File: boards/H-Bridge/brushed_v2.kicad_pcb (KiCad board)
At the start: 2 copper layers, 58 parts, among them IC1 ISO1042QDWVQ1, IC2 MIC4606-1YML-TR, IC3 AD8410AWBRZ-RL, IC4 TC1108-3.3VDBTR, J1 V+, J2 V-, J3 Motor-, J4 Motor+, J5 CANBus, J6 Encoder, J7 Prog_Header, J8 UART, J9 12V+, Q1 NTBLS4D0N15MC, Q2 NTBLS4D0N15MC, Q3 NTBLS4D0N15MC, Q4 NTBLS4D0N15MC, U1 STM32F103C8Tx, U2 LSF0102DCUR, U3 LSF0102DCUR

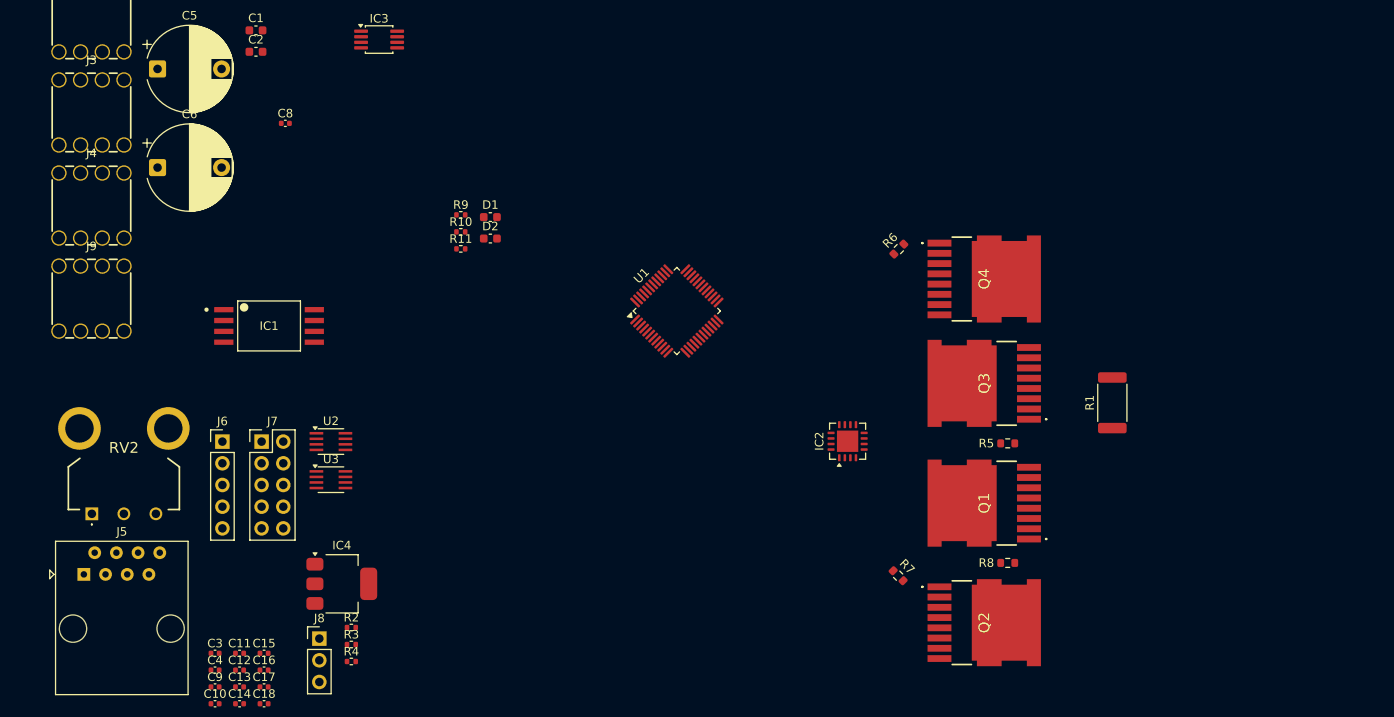
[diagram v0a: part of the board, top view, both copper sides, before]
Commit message: did some layout
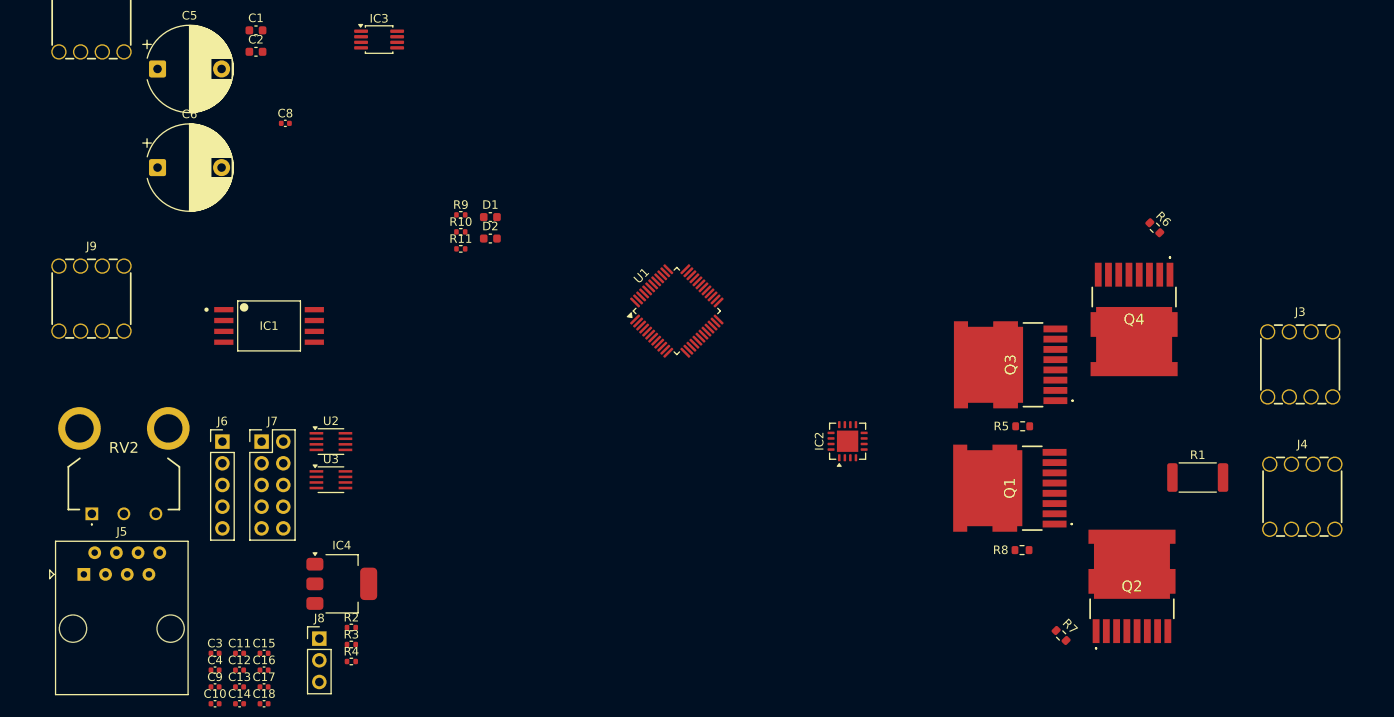
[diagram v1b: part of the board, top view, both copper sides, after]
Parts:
- moved J4 145.8 mm to (224.5, 116.8)
- moved J3 144.6 mm to (224.2, 101.2)
- moved R6 30.1 mm to (207.2, 85.2), turned to -45 degrees
- moved R7 20.3 mm to (196.2, 133.0)
- moved Q4 18.2 mm to (204.8, 96.0), turned to 180 degrees
- moved Q2 17.8 mm to (204.6, 127.2), turned to 0 degrees
- moved R1 13.3 mm to (212.2, 114.5), turned to 0 degrees
- moved Q3 3.78 mm to (190.3, 101.3)
- moved Q1 3.47 mm to (190.2, 115.8)
- moved R5 2.66 mm to (191.8, 108.5)
- moved R8 2.25 mm to (191.7, 123.0)
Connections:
- IC3 pad 1: /High Voltage&Sense/BHS -> /High Voltage&Sense/SHUNT-
- IC3 pad 8: /High Voltage&Sense/SHUNT+ -> /High Voltage&Sense/AHS
- J4 pad 1: /High Voltage&Sense/AHS -> /High Voltage&Sense/SHUNT-
- R1 pad 1: /High Voltage&Sense/SHUNT+ -> /High Voltage&Sense/AHS
- R1 pad 2: /High Voltage&Sense/BHS -> /High Voltage&Sense/SHUNT-

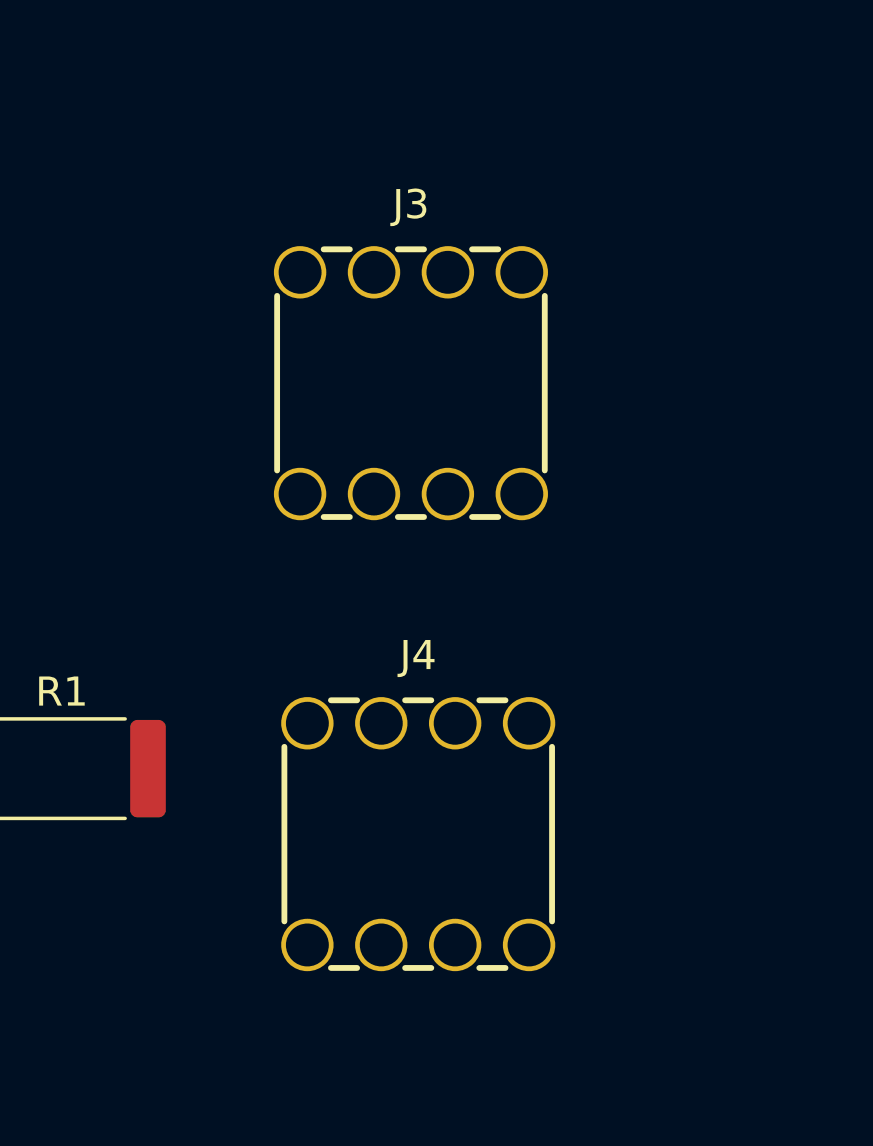
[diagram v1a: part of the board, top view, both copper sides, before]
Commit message: thought some more
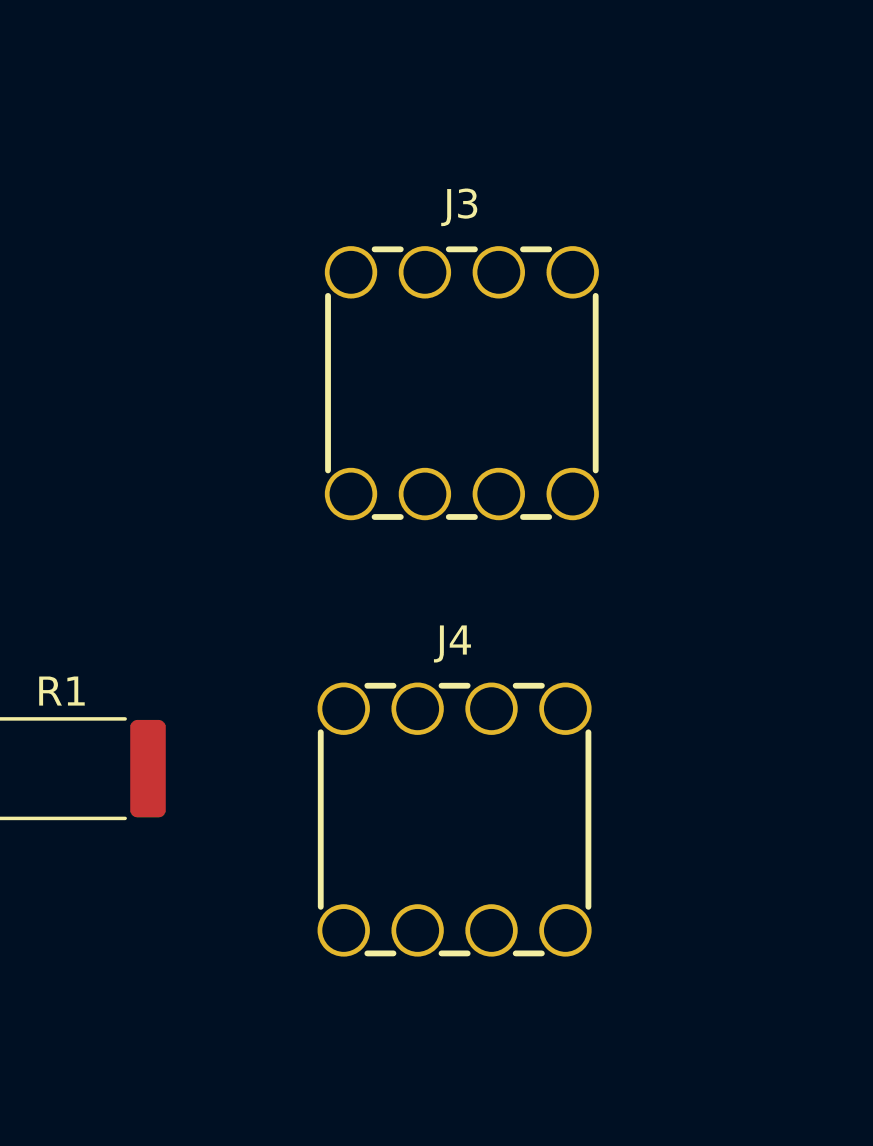
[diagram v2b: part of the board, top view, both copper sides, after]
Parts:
- moved J3 1.75 mm to (226.0, 101.2)
- moved J4 1.35 mm to (225.8, 116.2)
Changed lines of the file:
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@@
 	(footprint "ThreadedConnector:WP-BUTR_7460307"
 		(layer "F.Cu")
-		(at 224.5 116.75)
+		(at 225.75 116.25)
 		(property "Reference" "J4"
 			(at 0 -6.135 0)
@@
 	(footprint "ThreadedConnector:WP-BUTR_7460307"
 		(layer "F.Cu")
-		(at 224.25 101.25)
+		(at 226 101.25)
 		(property "Reference" "J3"
 			(at 0 -6.135 0)
